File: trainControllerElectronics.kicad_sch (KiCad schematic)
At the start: 35 parts, among them J1 0541324062, J2 USB4135-GF-A, J3 B2B-PH-K-S, J4 Pin header 2.54 1x03, J5 Pin socket 2.54 1x03, Q1 BSS670S2LH6327XTSA1, SW1 PTS647SM38SMTR2 LFS, SW10 PTS647SM38SMTR2 LFS, SW11 PTS647SM38SMTR2 LFS, SW12 PTS647SM38SMTR2 LFS, SW2 PTS647SM38SMTR2 LFS, SW3 PTS647SM38SMTR2 LFS, SW4 PTS647SM38SMTR2 LFS, SW5 PTS647SM38SMTR2 LFS, SW6 PTS647SM38SMTR2 LFS, SW7 PTS647SM38SMTR2 LFS, SW8 PTS647SM38SMTR2 LFS, SW9 PTS647SM38SMTR2 LFS, U1 CD74HC4067M96, U2 ZXM64P03XTA, U3 MCP73831T-2ACI/OT

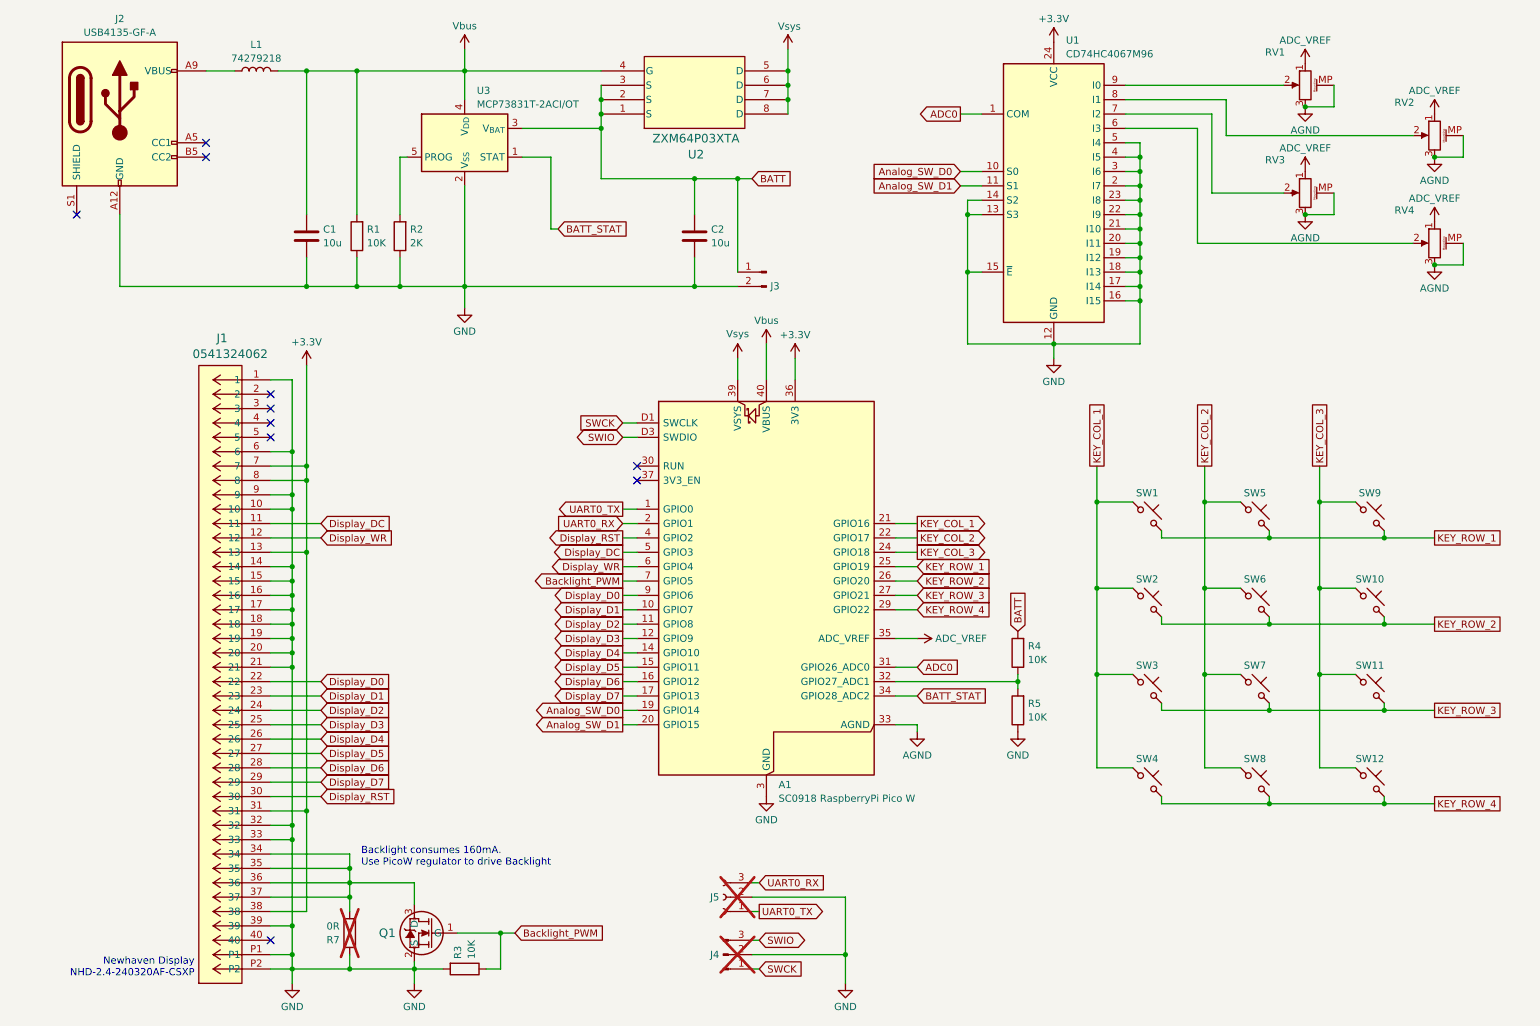
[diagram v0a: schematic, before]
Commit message: PCB ready
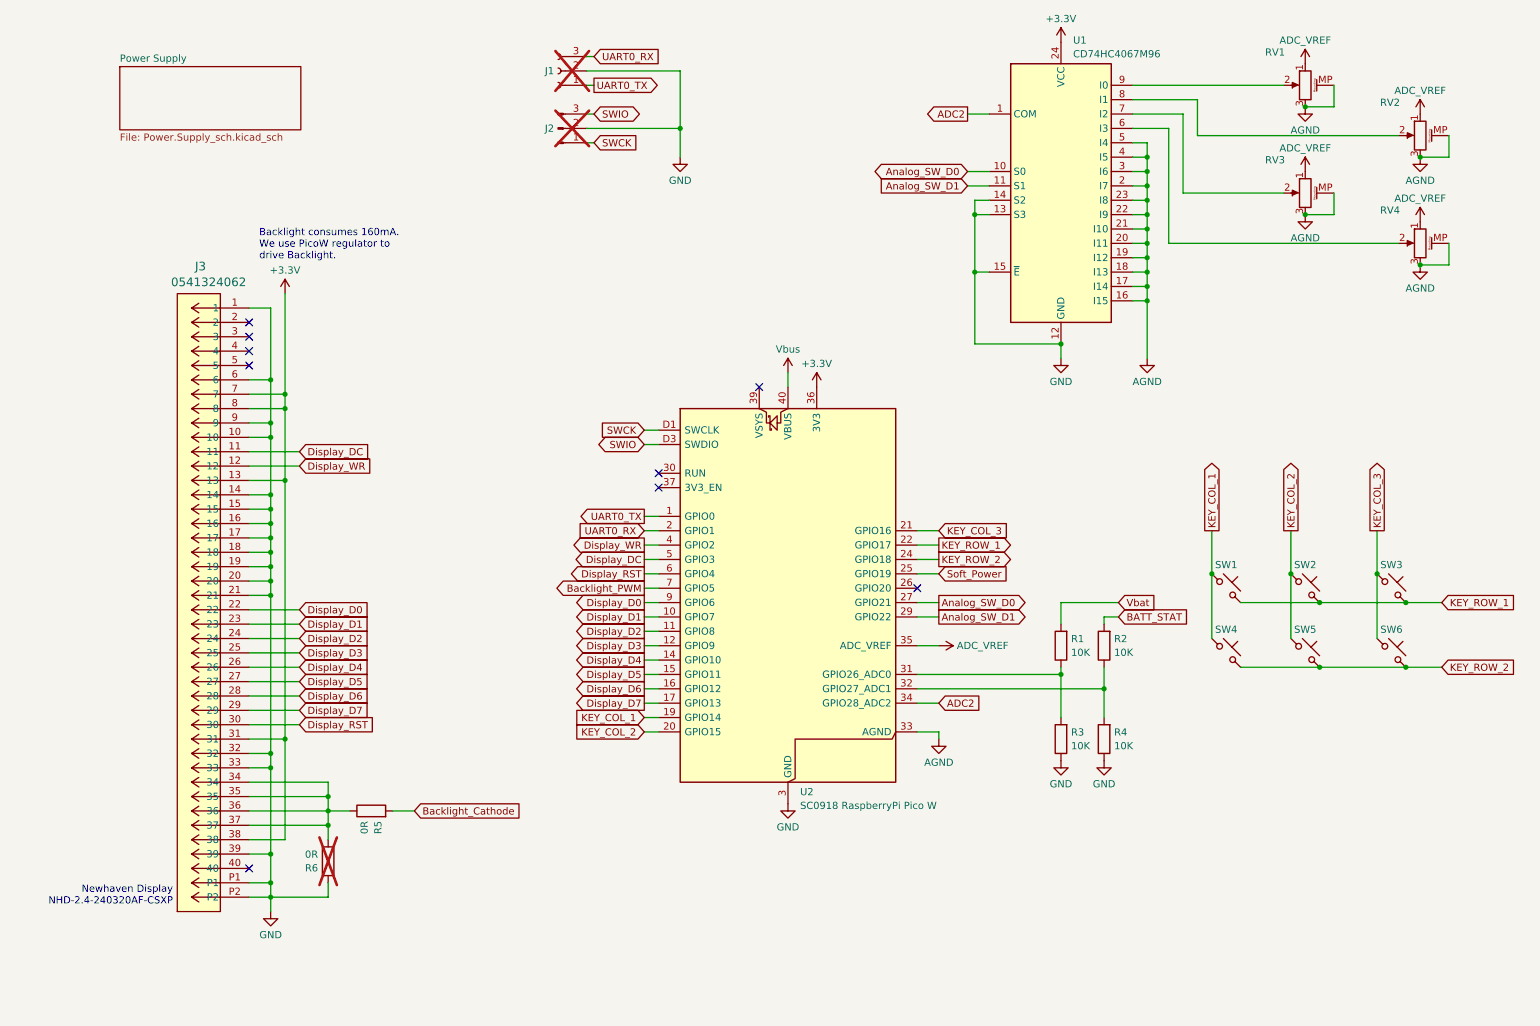
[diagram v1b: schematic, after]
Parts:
- removed C1, C2: 10u, Capacitor_SMD:C_0805_2012Metric_Pad1.18x1.45mm_HandSolder, symbol Device:C
- removed J2: USB4135-GF-A, Connector_USB:USB_C_Receptacle_GCT_USB4135-GF-A_6P_TopMnt_Horizontal, symbol Connector:USB_C_Receptacle_PowerOnly_6P
- removed J3: B2B-PH-K-S, Connector_JST:JST_PH_B2B-PH-K_1x02_P2.00mm_Vertical, symbol Connector:Conn_01x02_Pin
- removed L1: 74279218, Inductor_SMD:L_1206_3216Metric_Pad1.42x1.75mm_HandSolder, symbol Device:L
- removed Q1: BSS670S2LH6327XTSA1, BSS670S2L:PG-SOT23-3-5_INF, symbol BSS670S2L:BSS670S2LH6327XTSA1
- removed R1, R3: 10K, Resistor_SMD:R_0805_2012Metric_Pad1.20x1.40mm_HandSolder, symbol Device:R
- removed SW10, SW11, SW12, SW7, SW8, SW9: PTS647SM38SMTR2 LFS, Button_Switch_SMD:SW_SPST_PTS647_Sx38, symbol Switch:SW_Push_45deg
- removed U2: ZXM64P03XTA, SOIC8_ZXM64P03X_DIO, symbol ZXM64P03XTA:ZXM64P03XTA
- removed U3: MCP73831T-2ACI/OT, Package_TO_SOT_SMD:SOT-23-5, symbol Battery_Management:MCP73831-2-OT
- added R4: 10K, Resistor_SMD:R_0805_2012Metric_Pad1.20x1.40mm_HandSolder, symbol Device:R
- added R5: 0R, Resistor_SMD:R_0805_2012Metric_Pad1.20x1.40mm_HandSolder, symbol Device:R
- R2: value 2K -> 10K
- SW1, SW2, SW3, SW4, SW5, SW6: value PTS647SM38SMTR2 LFS -> 1825910-6; footprint Button_Switch_SMD:SW_SPST_PTS647_Sx38 -> Button_Switch_THT:SW_PUSH_6mm; Digikey part PTS647SM38SMTR2LFSCT-ND -> 450-1650-ND; Manufacturer С&K Components -> TE CONNECTIVITY; Manufacturer part PTS647SM38SMTR2 LFS -> 1825910-6
- renumbered J5 to J1, J4 to J2, J1 to J3, R4 to R1, R5 to R3, R7 to R6, A1 to U2
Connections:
- net AGND: now also U1.16 (I15), U1.17 (I14), U1.18 (I13), U1.19 (I12), U1.2 (I7), U1.20 (I11), U1.21 (I10), U1.22 (I9), U1.23 (I8), U1.3 (I6), U1.4 (I5), U1.5 (I4)
- net Analog_SW_D0: now also U2.27 (GPIO21); no longer U2.19 (GPIO14)
- net Analog_SW_D1: now also U2.29 (GPIO22); no longer U2.20 (GPIO15)
- net BATT_STAT: now also R2.2; no longer U2.34 (GPIO28_ADC2)
- net Display_RST: now also U2.6 (GPIO4); no longer U2.4 (GPIO2)
- net Display_WR: now also U2.4 (GPIO2); no longer U2.6 (GPIO4)
- net GND: now also R4.1; no longer R2.1, U1.16 (I15), U1.17 (I14), U1.18 (I13), U1.19 (I12), U1.2 (I7), U1.20 (I11), U1.21 (I10), U1.22 (I9), U1.23 (I8), U1.3 (I6), U1.4 (I5), U1.5 (I4)
- net KEY_COL_1: now also U2.19 (GPIO14); no longer SW2.1, SW3.1, U2.21 (GPIO16)
- net KEY_COL_2: now also SW2.1, U2.20 (GPIO15); no longer SW6.1, U2.22 (GPIO17)
- net KEY_COL_3: now also SW3.1, SW6.1, U2.21 (GPIO16); no longer U2.24 (GPIO18)
- net KEY_ROW_1: now also SW2.2, SW3.2, U2.22 (GPIO17); no longer SW5.2, U2.25 (GPIO19)
- net KEY_ROW_2: now also SW4.2, SW5.2, U2.24 (GPIO18); no longer SW2.2, U2.26 (GPIO20)
- net at J3.34, J3.35, J3.36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: now also R5.1
- net at R1.1, R3.2: now also U2.31 (GPIO26_ADC0); no longer U2.32 (GPIO27_ADC1)
- net ADC0 renamed ADC2
- net ADC2: now also U2.34 (GPIO28_ADC2); no longer U2.31 (GPIO26_ADC0)
- net BATT renamed Vbat
- removed net KEY_ROW_3: SW3.2, U2.27 (GPIO21)
- removed net KEY_ROW_4: SW4.2, U2.29 (GPIO22)
- net Vsys: no longer names the net of U2.39 (VSYS)
- new net: R2.1, R4.2, U2.32 (GPIO27_ADC1)
- new net Backlight_Cathode: R5.2
- new net Soft_Power: U2.25 (GPIO19)
- no-connect marks 10 -> 9
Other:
- added sheet Power Supply (Power.Supply_sch.kicad_sch)
- note added: "Backlight consumes 160mA. We use PicoW regulator to drive Backlight."
- note removed: "Backlight consumes 160mA. Use PicoW regulator to drive Backlight"
- moved on the sheet: J1, J2, J3, R1, R3, R6, RV2, RV4, U1, U2
